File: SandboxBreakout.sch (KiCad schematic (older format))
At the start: 7 parts

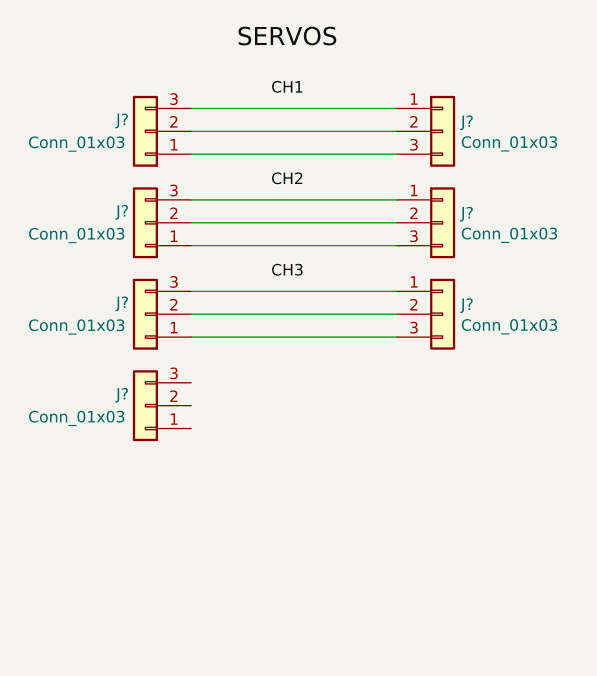
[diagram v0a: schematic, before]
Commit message: test commit
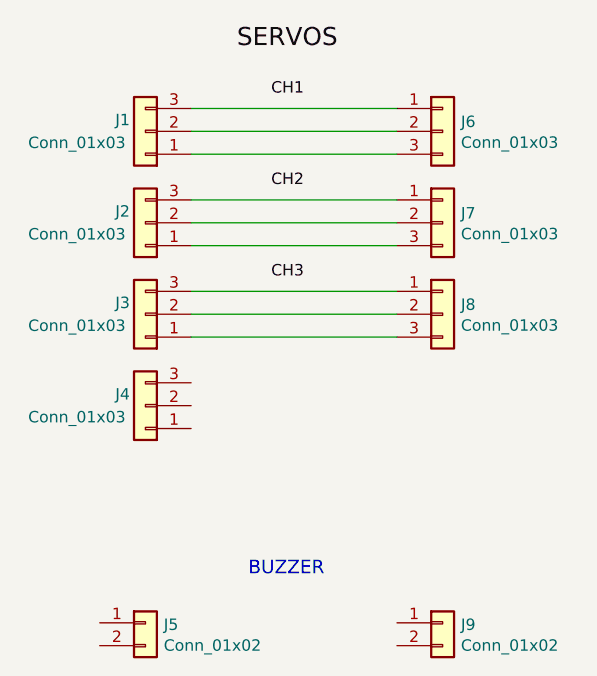
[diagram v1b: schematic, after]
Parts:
- added J5, J9: Conn_01x02, symbol Connector_Generic:Conn_01x02
- gave numbers to parts that had none: 7
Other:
- note added: "BUZZER"
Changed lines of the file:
@@
 	2700 1350 3600 1350
 $Comp
-L Connector_Generic:Conn_01x03 J?
+L Connector_Generic:Conn_01x03 J2
 U 1 1 616A49A7
 P 2500 1450
-F 0 "J?" H 2600 1400 50  0000 C CNN
+F 0 "J2" H 2600 1400 50  0000 C CNN
 F 1 "Conn_01x03" H 2800 1500 50  0000 C CNN
 F 2 "" H 2500 1450 50  0001 C CNN
@@
 $EndComp
 $Comp
-L Connector_Generic:Conn_01x03 J?
+L Connector_Generic:Conn_01x03 J7
 U 1 1 616A2D49
 P 3800 1450
-F 0 "J?" H 3880 1492 50  0000 L CNN
+F 0 "J7" H 3880 1492 50  0000 L CNN
 F 1 "Conn_01x03" H 3880 1401 50  0000 L CNN
 F 2 "" H 3800 1450 50  0001 C CNN
@@
 $EndComp
 $Comp
-L Connector_Generic:Conn_01x03 J?
+L Connector_Generic:Conn_01x03 J1
 U 1 1 616A1CEF
 P 2500 1050
-F 0 "J?" H 2600 1000 50  0000 C CNN
+F 0 "J1" H 2600 1000 50  0000 C CNN
 F 1 "Conn_01x03" H 2800 1100 50  0000 C CNN
 F 2 "" H 2500 1050 50  0001 C CNN
@@
 $EndComp
 $Comp
-L Connector_Generic:Conn_01x03 J?
+L Connector_Generic:Conn_01x03 J6
 U 1 1 616A09CD
 P 3800 1050
-F 0 "J?" H 3880 1092 50  0000 L CNN
+F 0 "J6" H 3880 1092 50  0000 L CNN
 F 1 "Conn_01x03" H 3880 1001 50  0000 L CNN
 F 2 "" H 3800 1050 50  0001 C CNN
@@
 $EndComp
 $Comp
-L Connector_Generic:Conn_01x03 J?
+L Connector_Generic:Conn_01x03 J3
 U 1 1 616A9CD6
 P 2500 1850
-F 0 "J?" H 2600 1800 50  0000 C CNN
+F 0 "J3" H 2600 1800 50  0000 C CNN
 F 1 "Conn_01x03" H 2800 1900 50  0000 C CNN
 F 2 "" H 2500 1850 50  0001 C CNN
@@
 $EndComp
 $Comp
-L Connector_Generic:Conn_01x03 J?
+L Connector_Generic:Conn_01x03 J8
 U 1 1 616A9FAA
 P 3800 1850
-F 0 "J?" H 3880 1892 50  0000 L CNN
+F 0 "J8" H 3880 1892 50  0000 L CNN
 F 1 "Conn_01x03" H 3880 1801 50  0000 L CNN
 F 2 "" H 3800 1850 50  0001 C CNN
@@
 CH3
 $Comp
-L Connector_Generic:Conn_01x03 J?
+L Connector_Generic:Conn_01x03 J4
 U 1 1 616AC14C
 P 2500 2250
-F 0 "J?" H 2600 2200 50  0000 C CNN
+F 0 "J4" H 2600 2200 50  0000 C CNN
 F 1 "Conn_01x03" H 2800 2300 50  0000 C CNN
 F 2 "" H 2500 2250 50  0001 C CNN
@@
 	-1   0    0    1
 $EndComp
+$Comp
+L Connector_Generic:Conn_01x02 J9
+U 1 1 616C2167
+P 3800 3200
+F 0 "J9" H 3880 3192 50  0000 L CNN
+F 1 "Conn_01x02" H 3880 3101 50  0000 L CNN
+F 2 "" H 3800 3200 50  0001 C CNN
+F 3 "~" H 3800 3200 50  0001 C CNN
+	1    3800 3200
+	1    0    0    -1
+$EndComp
+$Comp
+L Connector_Generic:Conn_01x02 J5
+U 1 1 616C163A
+P 2500 3200
+F 0 "J5" H 2580 3192 50  0000 L CNN
+F 1 "Conn_01x02" H 2580 3101 50  0000 L CNN
+F 2 "" H 2500 3200 50  0001 C CNN
+F 3 "~" H 2500 3200 50  0001 C CNN
+	1    2500 3200
+	1    0    0    -1
+$EndComp
+Text Notes 2950 3000 0    59   ~ 0
+BUZZER
 $EndSCHEMATC
